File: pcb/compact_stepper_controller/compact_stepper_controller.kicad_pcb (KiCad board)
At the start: 4 copper layers, 99 x 89 mm, 40 parts, among them J1 Screw Terminal, J10 1x2 Pin, J11 1x4 Pin, J12 Screw Terminal, J13 Screw Terminal, J14 Screw Terminal, J15 Conn_01x06_Pin, J16 Screw Terminal, J17 Screw Terminal, J2 1x4 Pin, J3 1x4 Pin, J4 1x4 Pin, J5 1x4 Pin, J6 1x2 Pin, J7 1x2 Pin, J8 1x2 Pin, J9 1x4 Pin, SW1 Switch, SW2 Switch, SW3 Switch, SW4 Switch, SW5 Switch, SW6 Switch, SW7 Switch, SW8 Switch

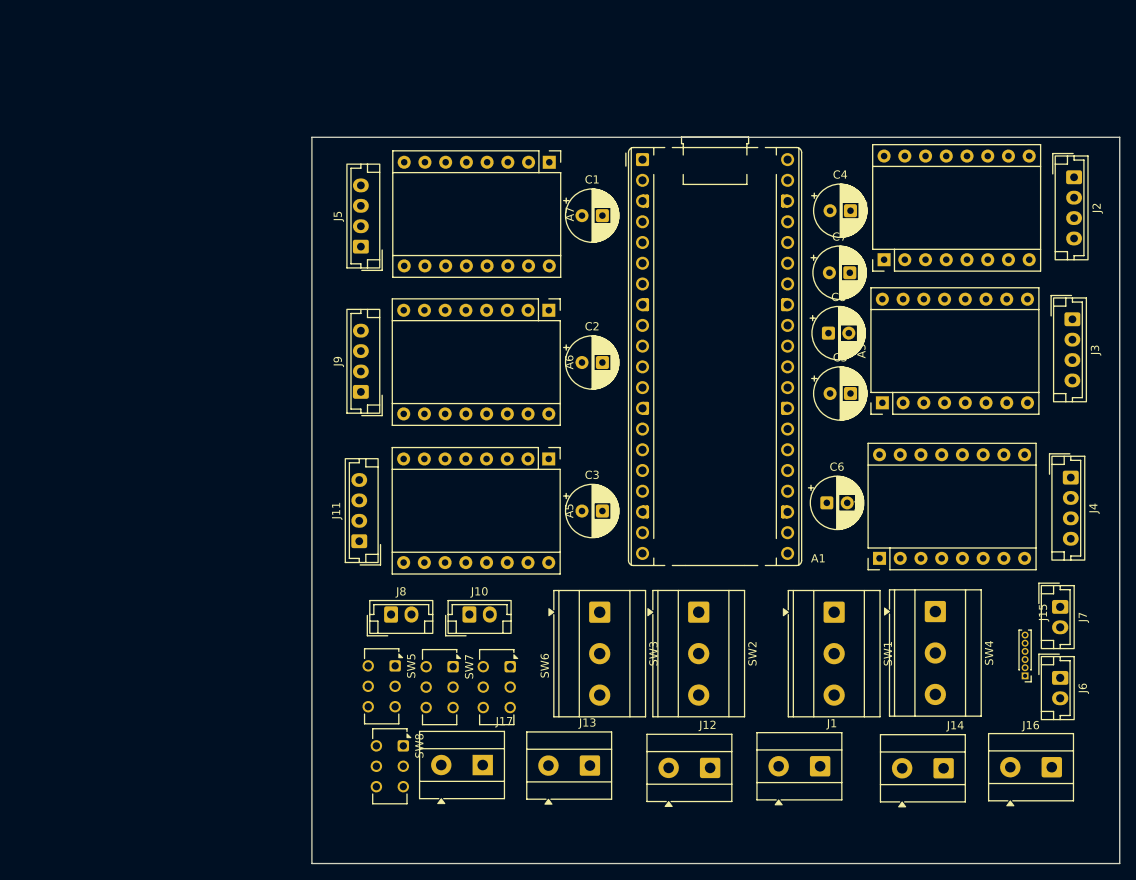
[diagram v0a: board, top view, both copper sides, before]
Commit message: V0.1 Compact PCB Done
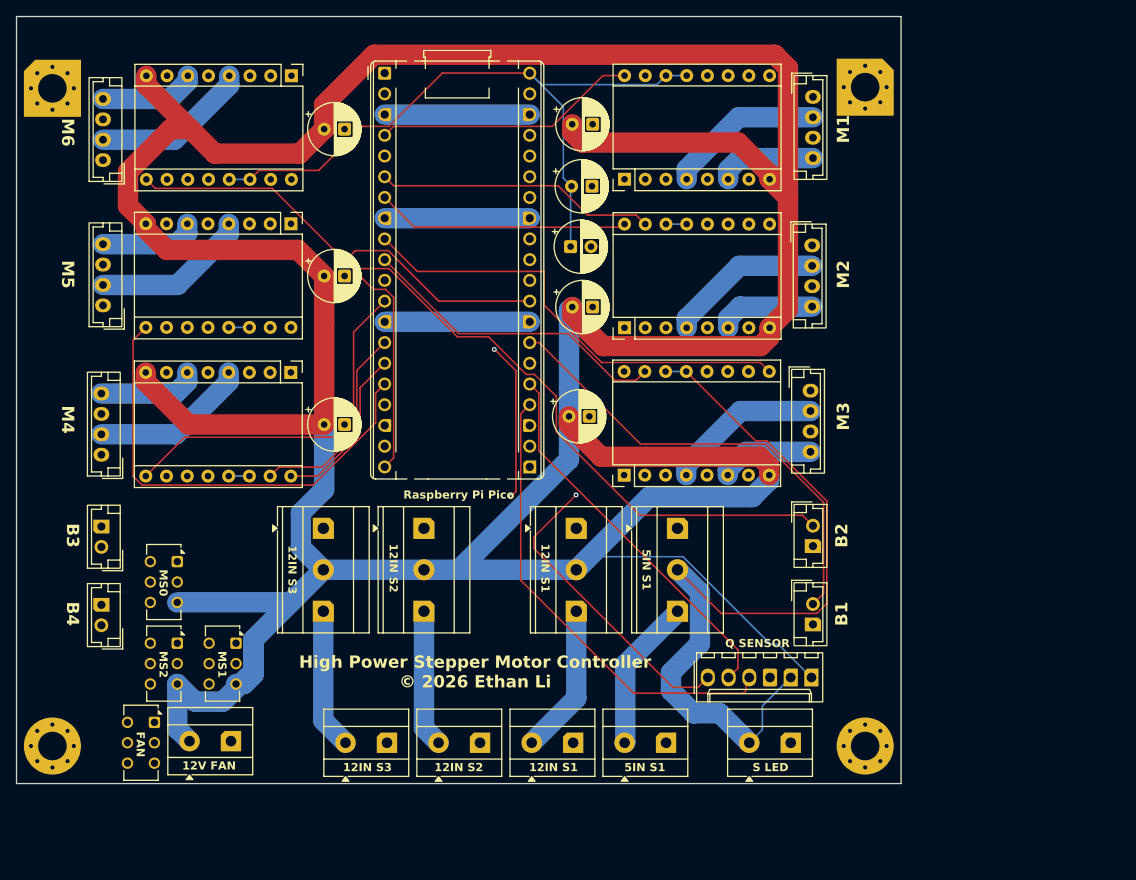
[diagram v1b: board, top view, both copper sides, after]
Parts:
- added REF**: MountingHole_3.5mm_Pad_Via, MountingHole:MountingHole_3.5mm_Pad_Via, F.Cu at (192.0, 62.3)
- added REF**: MountingHole_3.5mm_Pad_Via, MountingHole:MountingHole_3.5mm_Pad_Via, F.Cu at (92.4, 62.4)
- added REF**: MountingHole_3.5mm_Pad_Via, MountingHole:MountingHole_3.5mm_Pad_Via, F.Cu at (192.0, 143.0)
- added REF**: MountingHole_3.5mm_Pad_Via, MountingHole:MountingHole_3.5mm_Pad_Via, F.Cu at (92.4, 143.0)
- J15: footprint Connector_PinHeader_1.00mm:PinHeader_1x06_P1.00mm_Vertical -> Connector_Molex:Molex_KK-254_AE-6410-06A_1x06_P2.54mm_Vertical
- Raspberry Pi Pico : renamed from A1
- moved J10 45.9 mm to (98.4, 118.6), turned to 90 degrees
- moved J15 38.9 mm to (172.7, 134.6), turned to 0 degrees
- moved J8 35.5 mm to (98.4, 128.2), turned to 90 degrees
- moved SW3 35.4 mm to (125.6, 116.3)
- moved SW2 35.2 mm to (137.9, 116.3)
- moved J14 34.2 mm to (162.5, 142.6)
- moved SW7 33.9 mm to (107.7, 130.4)
- moved SW6 33.7 mm to (114.9, 130.4)
- moved J4 33.6 mm to (185.3, 99.5)
- moved J2 33.5 mm to (185.6, 63.5)
- moved C6 33.3 mm to (155.7, 102.6)
- moved C7 33.3 mm to (156.0, 74.4)
- moved C3 33.3 mm to (125.7, 103.6)
- moved C1 33.3 mm to (125.7, 67.4)
- moved C2 33.3 mm to (125.7, 85.4)
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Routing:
- net Net-(A1-AGND): track 0.00 -> 850.7 mm
- net Net-(A2-VMOT): track 0.00 -> 512.4 mm
- net Net-(A1-VBUS): track 0.00 -> 269.4 mm
- net Net-(A2-M0): track 0.00 -> 189.7 mm
- net Net-(A2-M1): track 0.00 -> 187.0 mm
- net Net-(A2-M2): track 0.00 -> 180.5 mm
- net Net-(A1-GPIO26_ADC0): track 0.00 -> 128.4 mm
- net Net-(A1-GPIO27_ADC1): track 0.00 -> 108.3 mm
- net Net-(A1-GPIO22): track 0.00 -> 98.3 mm
- net Net-(A1-GPIO3): track 0.00 -> 81.7 mm
- net Net-(A1-GPIO17): track 0.00 -> 61.3 mm, vias 0 -> 2
- net Net-(A1-GPIO15): track 0.00 -> 57.5 mm
- net Net-(A1-GPIO12): track 0.00 -> 57.4 mm
- net Net-(A1-GPIO18): track 0.00 -> 57.2 mm
- net Net-(A1-GPIO21): track 0.00 -> 57.1 mm
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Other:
- board size 99 x 89 mm -> 108.4 x 94 mm
- board text added: "12IN S1"
- board text added: "12IN S2"
- board text added: "12IN S3"
- board text added: "12V FAN"
- board text added: "5IN S1"
- board text added: "B1"
- board text added: "B2"
- board text added: "B3"
- board text added: "B4"
- board text added: "FAN"
- board text added: "High Power Stepper Motor Controller © 2026 Ethan Li"
- board text added: "M1"
- board text added: "M2"
- board text added: "M3"
- board text added: "M4"
- board text added: "M5"
- board text added: "M6"
- board text added: "MS0"
- board text added: "MS1"
- board text added: "MS2"
- board text added: "Q SENSOR"
- board text added: "Raspberry Pi Pico"
- board text added: "S LED"
